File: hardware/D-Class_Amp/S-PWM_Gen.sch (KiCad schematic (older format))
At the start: 10 parts, among them U201 Opamp_Dual_Generic, U202 Comparator_Dual_Generic

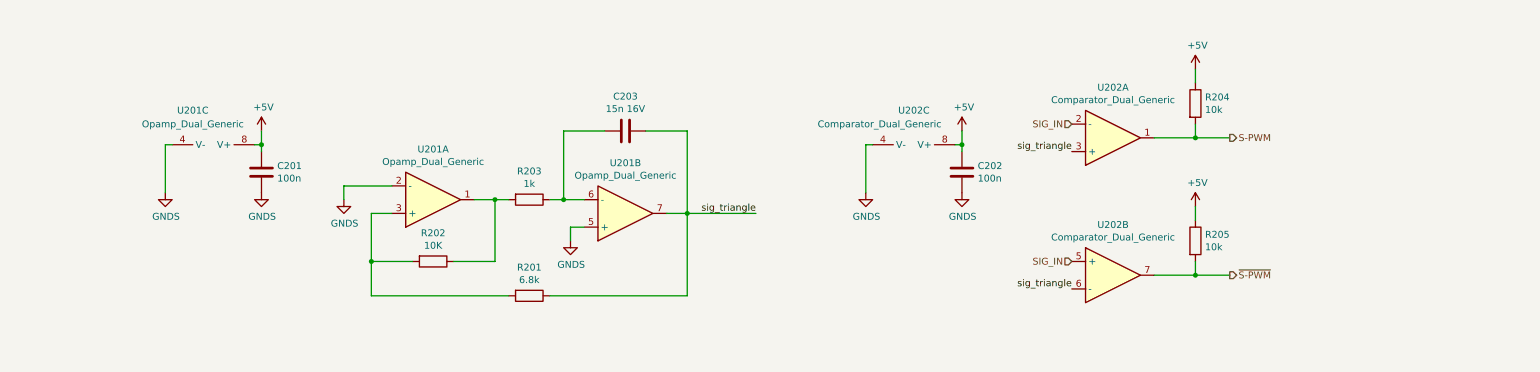
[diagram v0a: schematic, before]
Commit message: edits
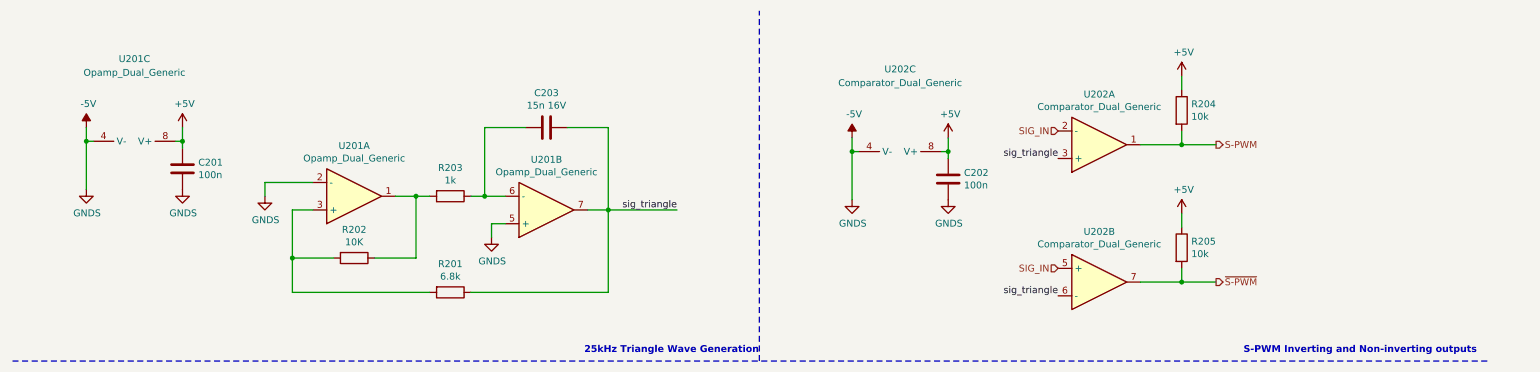
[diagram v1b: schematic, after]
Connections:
- net GNDS renamed -5V
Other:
- note added: "25kHz Triangle Wave Generation"
- note added: "S-PWM Inverting and Non-inverting outputs"
- moved on the sheet: C201, C202, C203, R201, R202, R203, R204, R205, U201A, U201B, U201C, U202A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
